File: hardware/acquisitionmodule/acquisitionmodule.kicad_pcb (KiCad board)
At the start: 2 copper layers, 57.8 x 38.1 mm, 11 parts, among them J1 Conn_Coaxial, J2 USB_B_Mini, J3 Conn_Coaxial, U1 LM358, U2 LM358

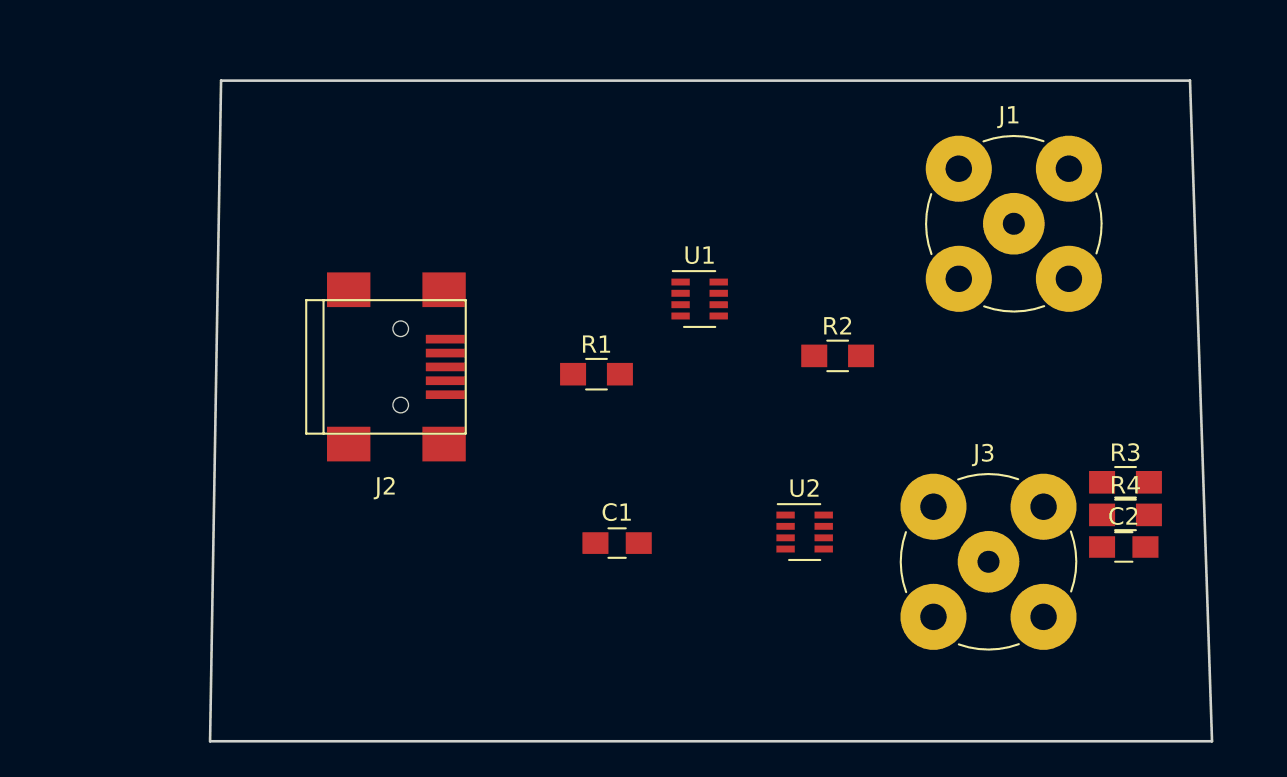
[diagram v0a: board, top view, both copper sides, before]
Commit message: changes in prive libs
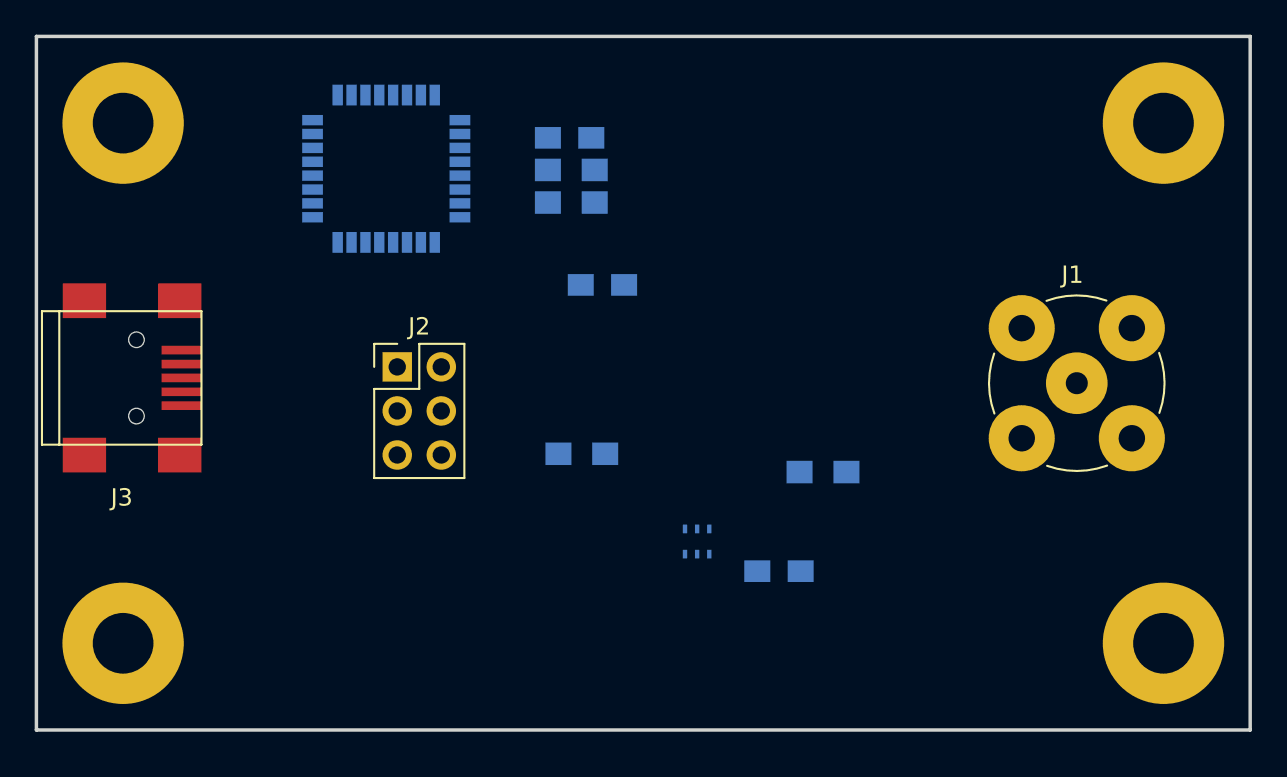
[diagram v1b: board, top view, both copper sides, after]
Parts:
- added C3: C, Capacitors_SMD:C_0805_HandSoldering, B.Cu at (152.8, 110.8)
- added REF**: MountingHole_3.5mm_Pad, Mounting_Holes:MountingHole_3.5mm_Pad, F.Cu at (175.0, 85.0)
- added REF**: MountingHole_3.5mm_Pad, Mounting_Holes:MountingHole_3.5mm_Pad, F.Cu at (175.0, 115.0)
- added REF**: MountingHole_3.5mm_Pad, Mounting_Holes:MountingHole_3.5mm_Pad, F.Cu at (115.0, 115.0)
- added REF**: MountingHole_3.5mm_Pad, Mounting_Holes:MountingHole_3.5mm_Pad, F.Cu at (115.0, 85.0)
- C1, C2, R1, R2, R3, R4: moved to B.Cu
- J2: value USB_B_Mini -> AVR-ISP-6; footprint Connectors:USB_Mini-B -> Pin_Headers:Pin_Header_Straight_2x03_Pitch2.54mm
- J3: value Conn_Coaxial -> USB_B_Mini; footprint Connectors:bnc-ci -> Connectors:USB_Mini-B
- U1: value LM358 -> ADS1110; footprint TO_SOT_Packages_SMD:SOT-23-8 -> IonizationChamber:ADS1110; moved to B.Cu
- U2: value LM358 -> ATtiny88-AU; footprint TO_SOT_Packages_SMD:SOT-23-8 -> Housings_QFP:LQFP-32_7x7mm_Pitch0.8mm; moved to B.Cu
- moved J3 50.5 mm to (115.6, 99.7)
- moved C2 39.7 mm to (140.7, 85.9)
- moved R4 37.6 mm to (140.8, 87.7)
- moved R3 35.8 mm to (140.8, 89.6)
- moved U2 32.0 mm to (130.2, 87.6)
- moved C1 14.9 mm to (142.6, 94.3)
- moved U1 13.3 mm to (147.4, 108.4)
- moved J1 9.89 mm to (170.0, 100.0)
- moved R2 6.75 mm to (155.4, 105.1)
- moved R1 4.67 mm to (141.5, 104.1)
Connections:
- C2 pad 1: Net-(C2-Pad1) -> VCC
- J2 pad 1: (no net) -> Net-(J2-Pad1)
- J2 pad 2: (no net) -> VCC
- J2 pad 4: (no net) -> Net-(J2-Pad4)
- J2 pad 5: (no net) -> Net-(J2-Pad5)
- J2 pad 6: Net-(J2-Pad6) -> GND
- J3 pad 1: Net-(J3-Pad1) -> VCC
- J3 pad 2: GND -> (no net)
- R3 pad 1: Net-(J3-Pad1) -> VCC
- R3 pad 2: GND -> Net-(R3-Pad2)
- R4 pad 1: Net-(C2-Pad1) -> Net-(R3-Pad2)
- R4 pad 2: Net-(J3-Pad1) -> GND
- U1 pad 1: (no net) -> Net-(C1-Pad1)
- U1 pad 2: (no net) -> GND
- U1 pad 3: (no net) -> Net-(U1-Pad3)
- U1 pad 4: (no net) -> Net-(U1-Pad4)
- U1 pad 5: (no net) -> VCC
- U1 pad 6: (no net) -> Net-(R3-Pad2)
- U2 pad 5: (no net) -> Net-(U2-Pad21)
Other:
- board size 57.8 x 38.1 mm -> 70 x 40 mm
